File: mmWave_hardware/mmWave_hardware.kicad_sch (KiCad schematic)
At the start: 46 parts, among them J1 Conn_02x08_Top_Bottom, U1 IWRL6432BDBAAMFR, U2 W25Q128JVS, U3 AMS1117-3.3, U4 TPS628502QDRLRQ1, Y1 40.000

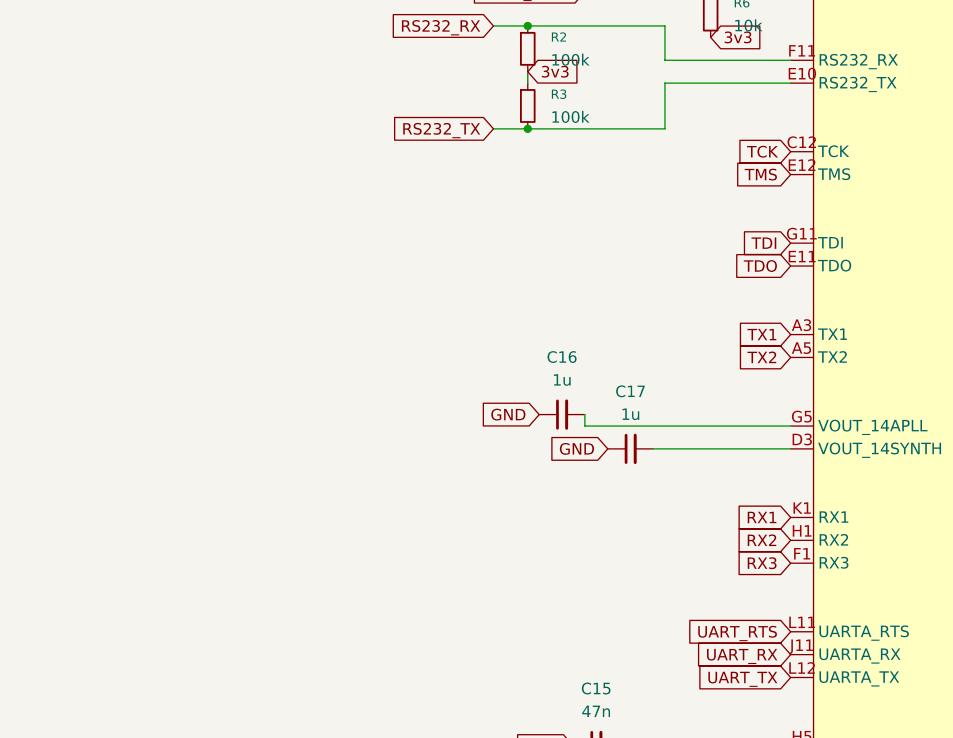
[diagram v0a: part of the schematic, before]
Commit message: antennaaaaaaaaaaaaaaaaaaaaa
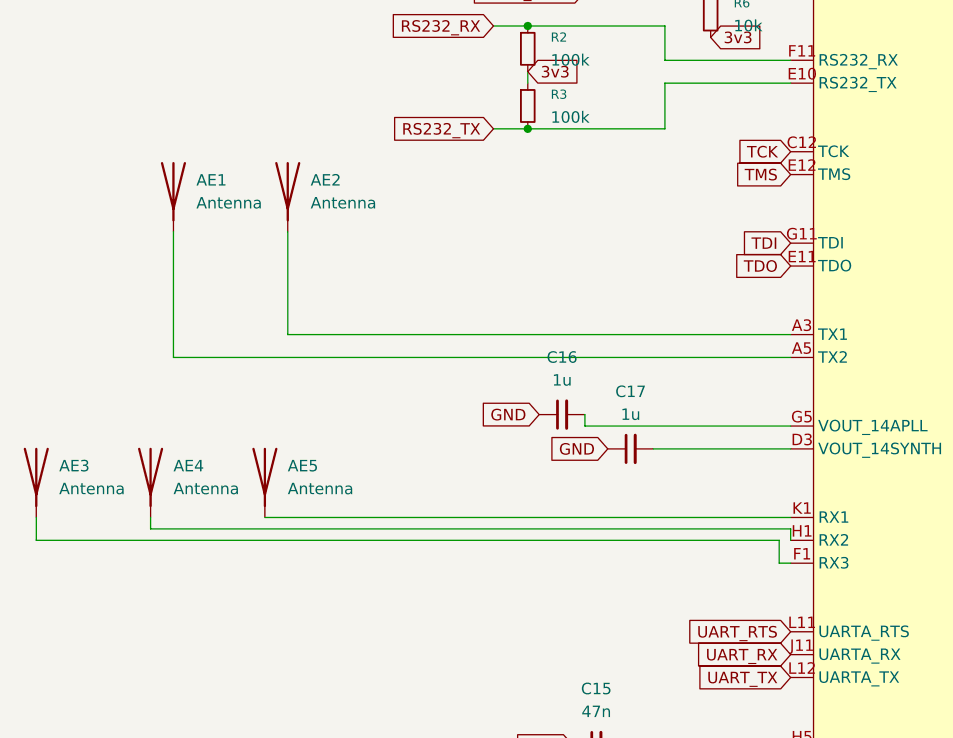
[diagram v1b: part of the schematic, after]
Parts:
- added AE1, AE2, AE3, AE4, AE5: Antenna, antennas:60GHz_microstrip_inset_patch, symbol Device:Antenna
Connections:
- net RX1: no longer names the net of U1.K1 (RX1)
- net RX1: now also AE5.1 (A)
- net RX2: no longer names the net of U1.H1 (RX2)
- net RX2: now also AE4.1 (A)
- net RX3: no longer names the net of U1.F1 (RX3)
- net RX3: now also AE3.1 (A)
- net TX1: no longer names the net of U1.A3 (TX1)
- net TX1: now also AE2.1 (A)
- net TX2: no longer names the net of U1.A5 (TX2)
- net TX2: now also AE1.1 (A)
